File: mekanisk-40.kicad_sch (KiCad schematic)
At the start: 125 parts, among them J1 USB_C_Receptacle_USB2.0, SW1 RST, SW2 RST, U2 USBLC6-2SC6, U3 STM32F072C8Tx, U4 XC6206PxxxMR-Regulator_Linear

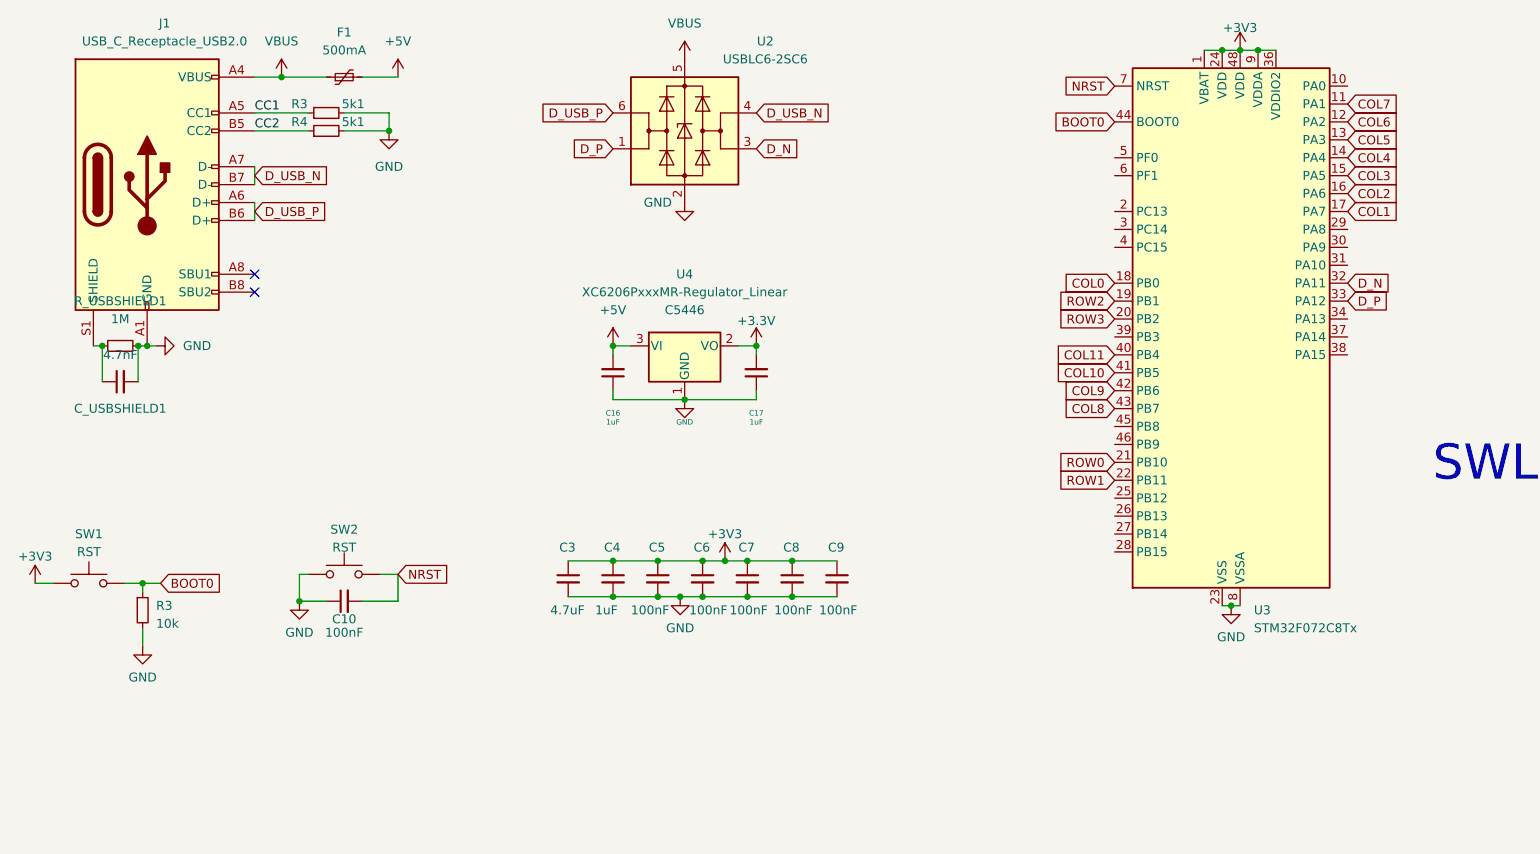
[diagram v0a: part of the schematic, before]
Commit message: first full design
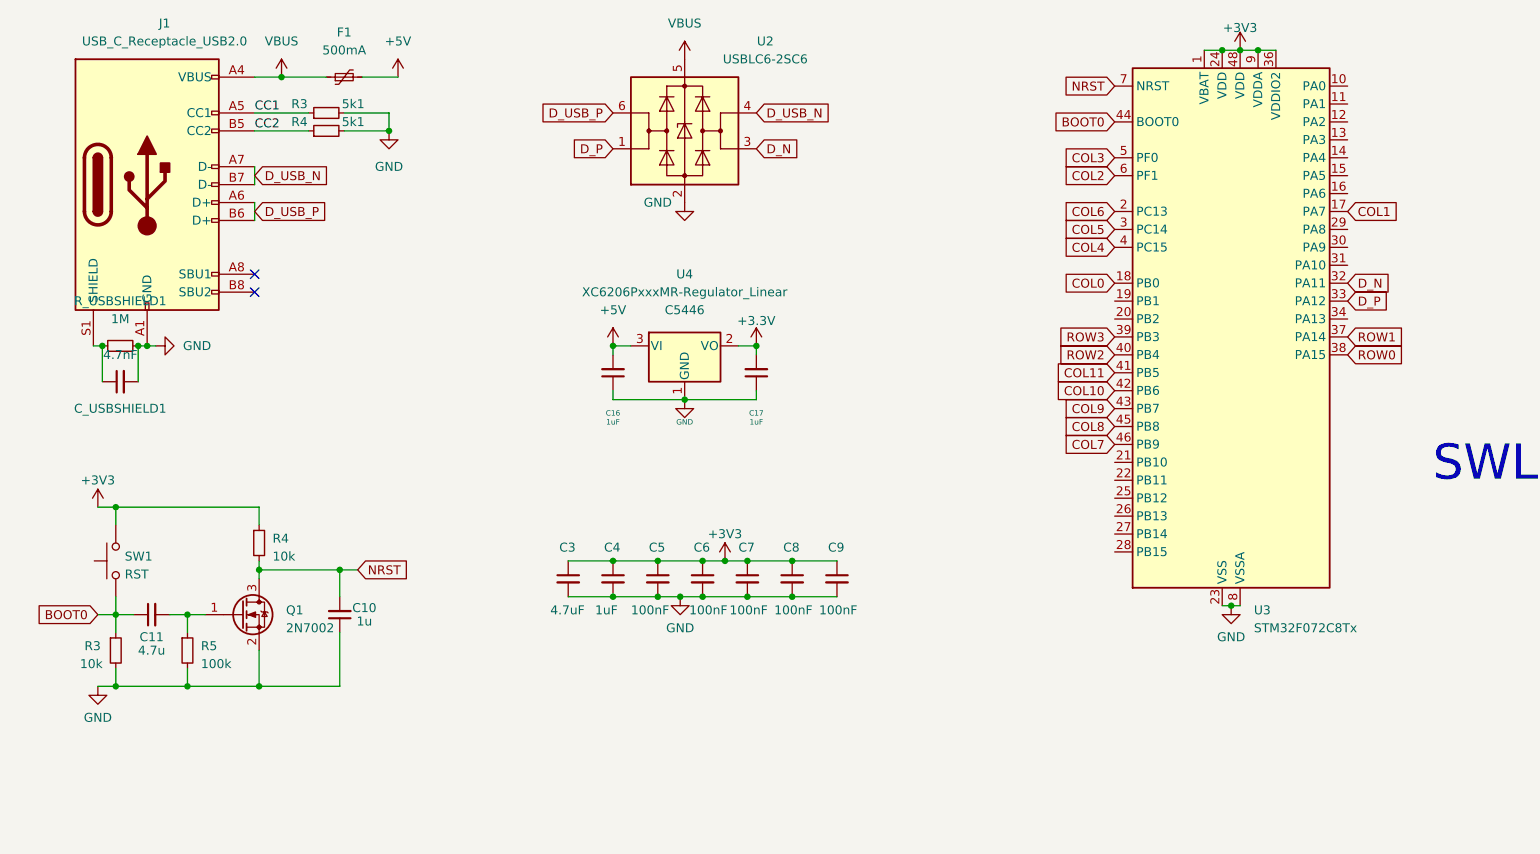
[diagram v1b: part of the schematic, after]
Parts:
- removed SW2: RST, Button_Switch_SMD:SW_SPST_SKQG_WithoutStem, symbol Switch:SW_Push
- added C11: 4.7u, Capacitor_SMD:C_0603_1608Metric, symbol Device:C_Small
- added Q1: 2N7002, Package_TO_SOT_SMD:SOT-23, symbol Transistor_FET:2N7002
- added R4: 10k, Resistor_SMD:R_0603_1608Metric, symbol Device:R_Small
- added R5: 100k, Resistor_SMD:R_0603_1608Metric, symbol Device:R_Small
- C10: value 100nF -> 1u
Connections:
- net +3V3: now also SW1.2, R4.1; no longer SW1.1
- net BOOT0: now also SW1.1, C11.1; no longer SW1.2
- net COL10: now also U3.42 (PB6); no longer U3.41 (PB5)
- net COL11: now also U3.41 (PB5); no longer U3.40 (PB4)
- net COL2: now also U3.6 (PF1); no longer U3.16 (PA6)
- net COL3: now also U3.5 (PF0); no longer U3.15 (PA5)
- net COL4: now also U3.4 (PC15); no longer U3.14 (PA4)
- net COL5: now also U3.3 (PC14); no longer U3.13 (PA3)
- net COL6: now also U3.2 (PC13); no longer U3.12 (PA2)
- net COL7: now also U3.46 (PB9); no longer U3.11 (PA1)
- net COL8: now also U3.45 (PB8); no longer U3.43 (PB7)
- net COL9: now also U3.43 (PB7); no longer U3.42 (PB6)
- net GND: now also Q1.2 (S), R5.2
- net NRST: now also Q1.3 (D), R4.2
- net ROW0: now also U3.38 (PA15); no longer U3.21 (PB10)
- net ROW1: now also U3.37 (PA14); no longer U3.22 (PB11)
- net ROW2: now also U3.40 (PB4); no longer U3.19 (PB1)
- net ROW3: now also U3.39 (PB3); no longer U3.20 (PB2)
- new net: C11.2, Q1.1 (G), R5.1
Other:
- moved on the sheet: C10, R3, SW1

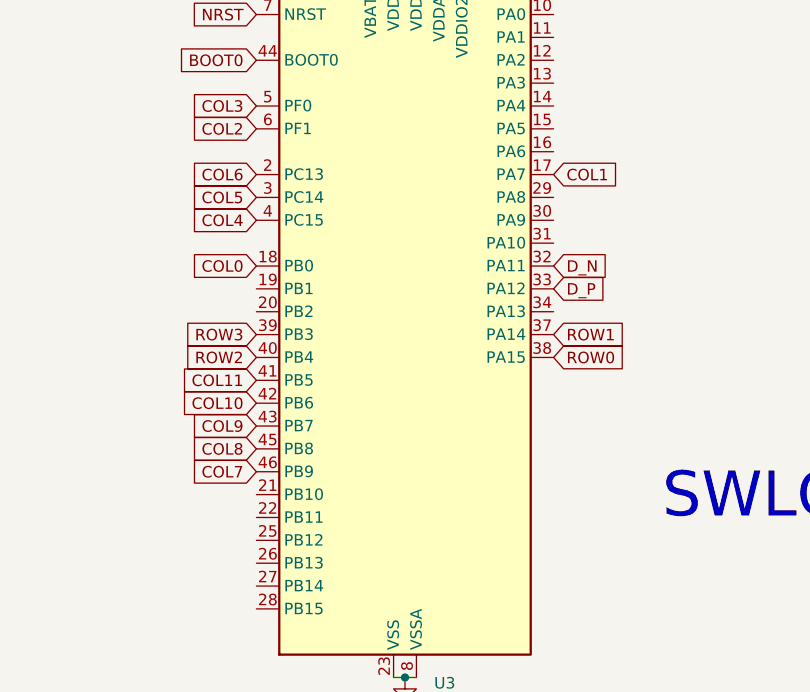
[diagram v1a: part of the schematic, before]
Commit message: slight routing cleanup
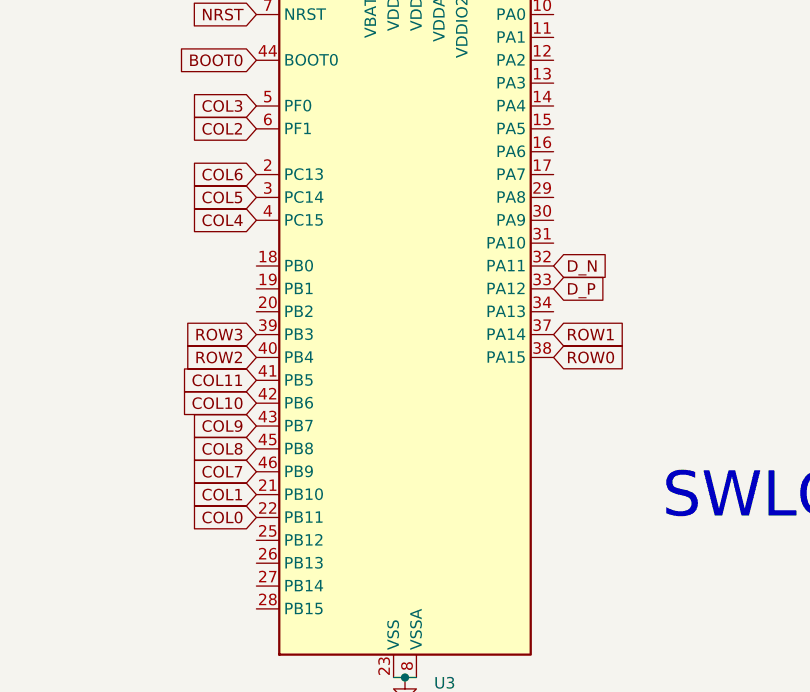
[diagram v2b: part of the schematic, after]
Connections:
- net COL0: now also U3.22 (PB11); no longer U3.18 (PB0)
- net COL1: now also U3.21 (PB10); no longer U3.17 (PA7)
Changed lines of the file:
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@@
     )
   )
-  (global_label "COL0" (shape input) (at 181.61 71.12 180) (fields_autoplaced)
+  (global_label "COL0" (shape input) (at 181.61 99.06 180) (fields_autoplaced)
     (effects (font (size 1.27 1.27)) (justify right))
-    (property "Intersheetrefs" "${INTERSHEET_REFS}" (at 173.8661 71.12 0)
+    (property "Intersheetrefs" "${INTERSHEET_REFS}" (at 173.8661 99.06 0)
       (effects (font (size 1.27 1.27)) (justify right) hide)
     )
@@
     )
   )
-  (global_label "COL1" (shape input) (at 214.63 60.96 0) (fields_autoplaced)
-    (effects (font (size 1.27 1.27)) (justify left))
-    (property "Intersheetrefs" "${INTERSHEET_REFS}" (at 222.3739 60.96 0)
-      (effects (font (size 1.27 1.27)) (justify left) hide)
+  (global_label "COL1" (shape input) (at 181.61 96.52 180) (fields_autoplaced)
+    (effects (font (size 1.27 1.27)) (justify right))
+    (property "Intersheetrefs" "${INTERSHEET_REFS}" (at 173.8661 96.52 0)
+      (effects (font (size 1.27 1.27)) (justify right) hide)
     )
   )
